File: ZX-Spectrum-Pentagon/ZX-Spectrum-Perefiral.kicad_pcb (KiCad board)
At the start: 2 copper layers, 4 parts, among them U1 74HC00

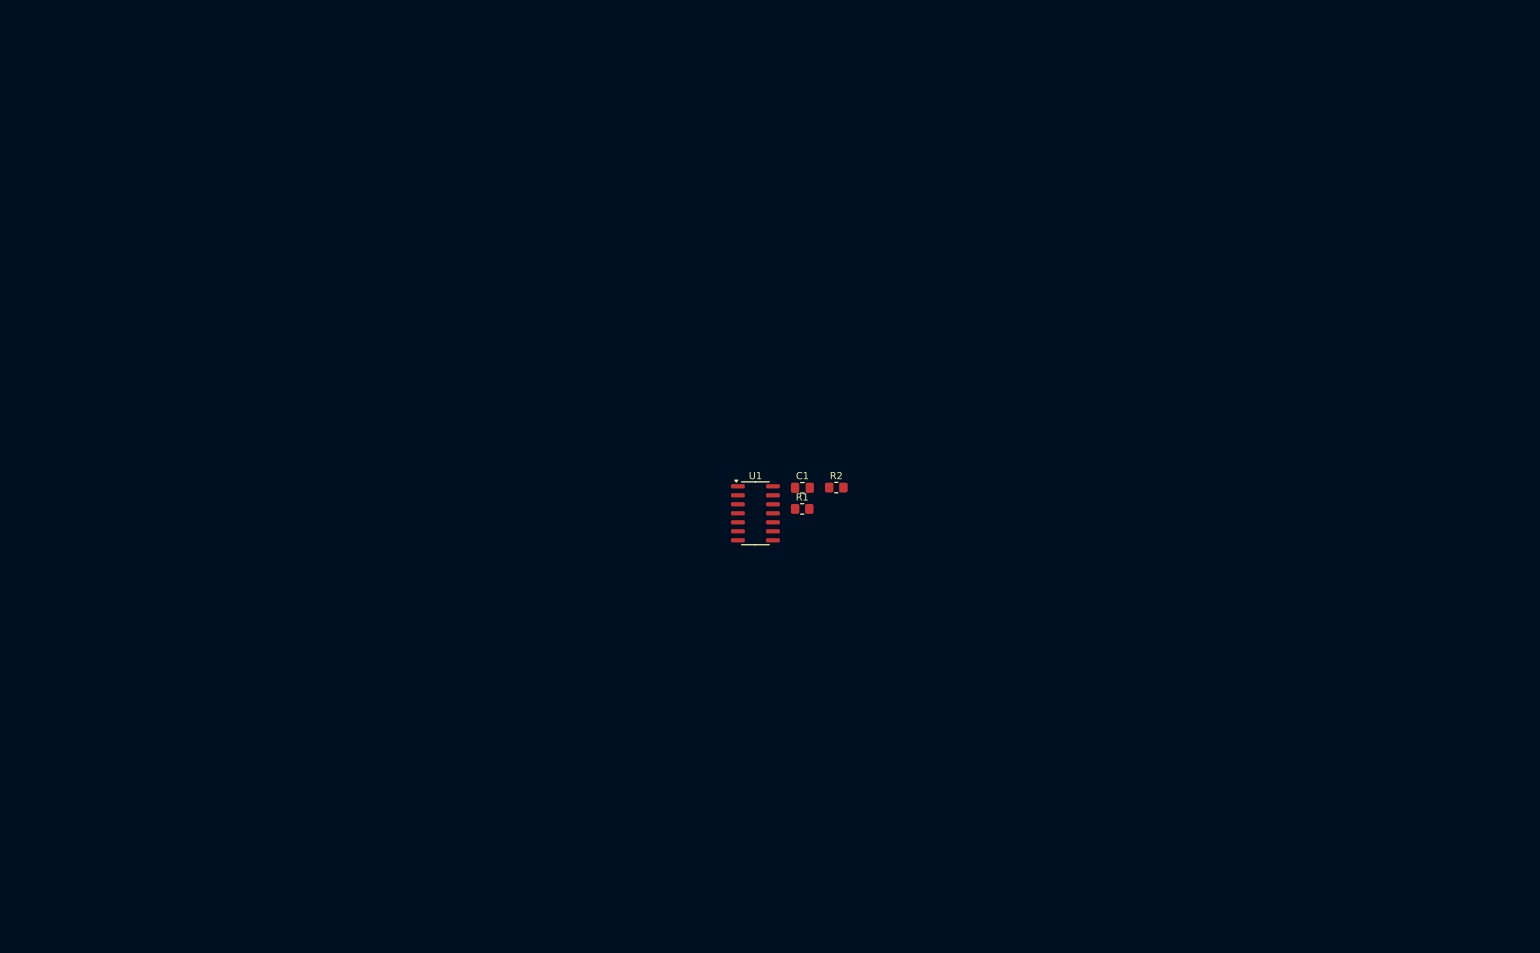
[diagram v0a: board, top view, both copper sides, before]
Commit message: add zxm_extrime_extension add 74XX283 to 74IEC start ZX-Spectrum-Perefiral project
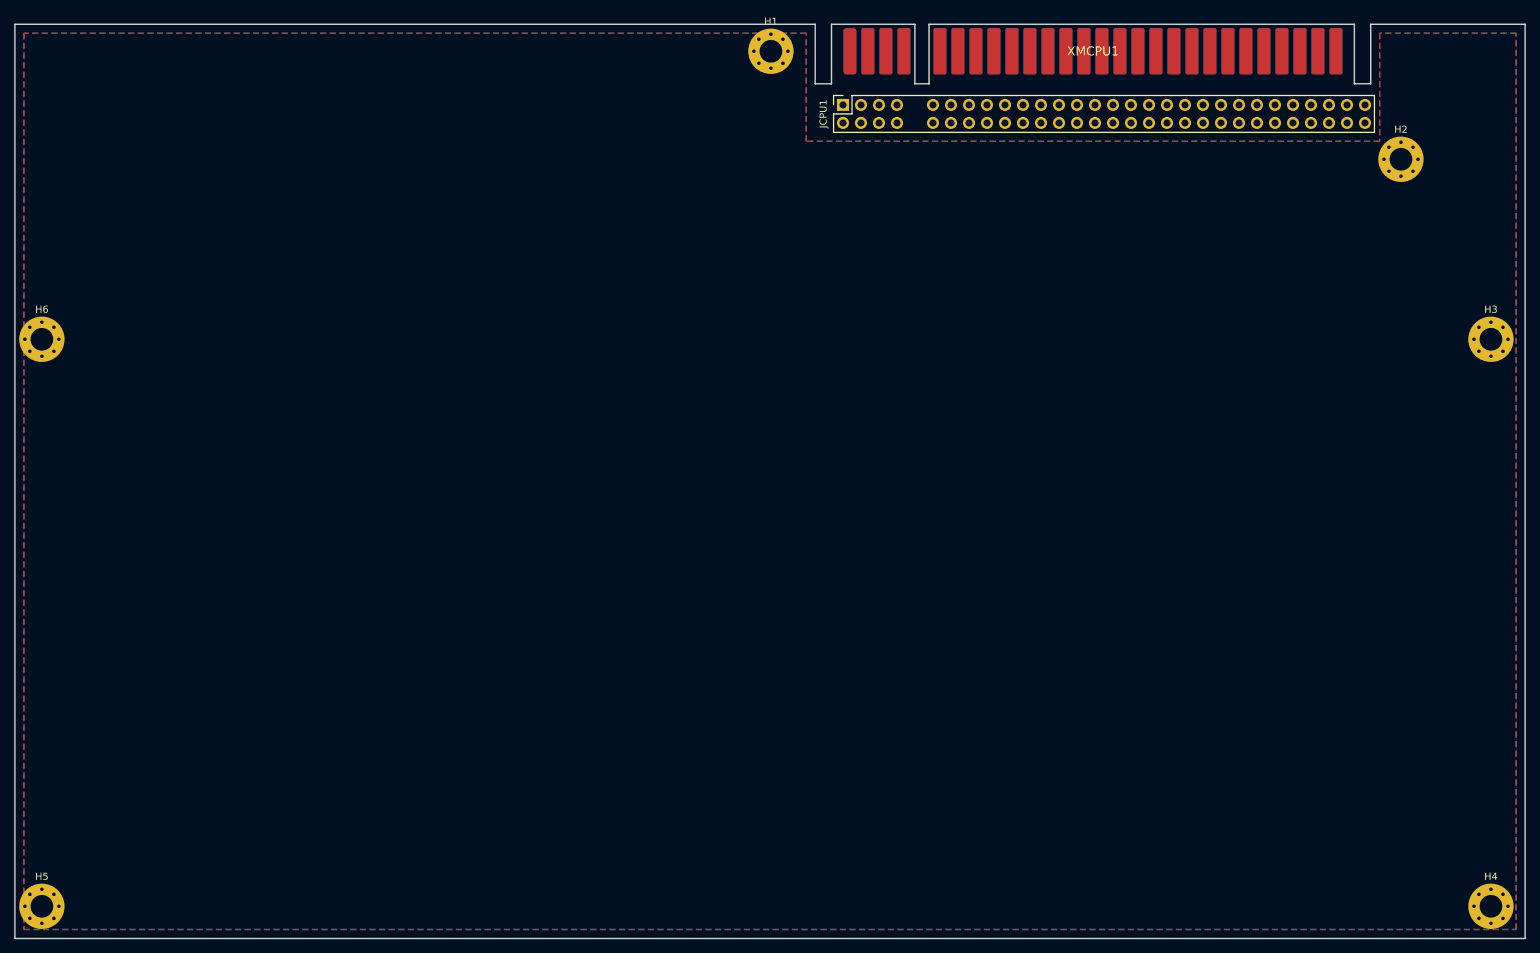
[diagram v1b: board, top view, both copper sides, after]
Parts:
- removed C1: C, Capacitor_SMD:C_0805_2012Metric_Pad1.18x1.45mm_HandSolder
- removed R1, R2: R, Resistor_SMD:R_0805_2012Metric_Pad1.20x1.40mm_HandSolder
- removed U1: 74HC00, Package_SO:SOIC-14_3.9x8.7mm_P1.27mm
- added H1: MountingHole_Pad, MountingHole:MountingHole_3.2mm_M3_Pad_Via, F.Cu at (127.0, 24.1)
- added H2: MountingHole_Pad, MountingHole:MountingHole_3.2mm_M3_Pad_Via, F.Cu at (215.9, 39.4)
- added H3: MountingHole_Pad, MountingHole:MountingHole_3.2mm_M3_Pad_Via, F.Cu at (228.6, 64.8)
- added H4: MountingHole_Pad, MountingHole:MountingHole_3.2mm_M3_Pad_Via, F.Cu at (228.6, 144.8)
- added H5: MountingHole_Pad, MountingHole:MountingHole_3.2mm_M3_Pad_Via, F.Cu at (24.1, 144.8)
- added H6: MountingHole_Pad, MountingHole:MountingHole_3.2mm_M3_Pad_Via, F.Cu at (24.1, 64.8)
- added JCPU1: TOP LEVEL, ZX-Spectrum-Pentagon:PinSocket_2x30_P2.54mm_Vertical, F.Cu at (174.0, 33.0)
- added XMCPU1: EDGE-28M5, ZX-Spectrum-Pentagon:EDGE_28M5-2.54, F.Cu at (172.4, 24.1)
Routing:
- added copper zone on F.Cu, net GND
- added copper zone on B.Cu, net VCC
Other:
- board outline added: 213.1 x 129 mm
- board text added: "EDGE connector position X=172.44 Y=24.13 BOARD connector position X=173.99 Y=33.02 Hole1: X=127 Y=24.13, Hole2: X=215.9 Y=39.37 Hole3: X=228.6 Y=64.77, Hole4: X=228.6 Y=144.78 Hole5: X=24.13 Y=144.78, Hole6: X=24.13 Y=64.77"
